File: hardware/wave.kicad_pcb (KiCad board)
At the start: 4 copper layers, 60 x 60 mm, 123 parts, among them J101 WAGO 2065-100, J102 WAGO 2065-100, J103 Cortex, J104 WAGO 2065-100, J105 WAGO 2065-100, J106 WAGO 2065-100, J107 WAGO 2065-100, J301 2x05_Horizontal, J401 2x05_Horizontal, J501 WAGO 2065-100, J502 WAGO 2065-100, Q201 IRF9358, SW101 SKSG, SW102 SKSG, U101 ATSAMD51J, U102 TPS78433QWDRBRQ1, U201 MA12070P, U301 THVD2442, U401 THVD2442, U501 74AHC1G125, Y101 32k768

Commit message: Update Library
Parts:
- FB101: value 47 Ohm -> ~
- FB201, FB202, FB203, FB204: value 50 Ohm -> ~
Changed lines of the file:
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@@
 			)
 		)
-		(property "Value" "50 Ohm"
+		(property "Value" "~"
 			(at 0 1.9 90)
 			(layer "F.Fab")
@@
 			)
 		)
-		(property "Value" "47 Ohm"
+		(property "Value" "~"
 			(at 0 2.9 0)
 			(layer "F.Fab")
@@
 			)
 		)
-		(property "Value" "50 Ohm"
+		(property "Value" "~"
 			(at 0 1.9 90)
 			(layer "F.Fab")
@@
 			)
 		)
-		(property "Value" "50 Ohm"
+		(property "Value" "~"
 			(at 0 1.9 90)
 			(layer "F.Fab")
@@
 		)
 		(group ""
-			(members "4532dc4e-f69d-412b-bc19-695d90100dcb" "8f0d22e3-918a-451d-a4a3-d23b9b599883"
-				"ae9bfc19-817d-4f4b-b84f-b22dd92c01e5" "bdaa4d0f-ab94-4c16-8f20-3c5ec3e83d21"
-				"f26a1357-79ae-4b96-a7f4-25831135af06"
+			(members "817afe4d-3ef8-4f34-841e-a1e0d13acd88" "8d5b3521-d299-4149-812d-e93ed26aa732"
+				"add876ea-4949-4e26-8186-7559bdf5a9eb" "b58fdfc9-b605-4197-b451-9f65004c44a9"
+				"c6308024-9361-453b-adb7-b5cdd279d357"
 			)
 		)
 		(group ""
-			(members "17461222-e6b8-4a40-a234-68067f321262" "96fa0783-c83b-424a-9582-f57065f0b73f"
-				"9e55e1cf-c869-4549-9032-91aab361908b" "9ef00dd0-bc50-46b7-b0af-3ca977389725"
-				"dabd2c8a-06ea-4384-a9f6-28d395331438"
+			(members "3d585795-267e-4acf-9233-fa6d3d19a673" "a58be4f5-7508-488d-900a-1671a0babb7c"
+				"bce2bd36-7243-4190-8a23-6d6964d44d4c" "e52a77fc-53a3-4bee-8404-ef76a262d8b0"
+				"fb6306f7-0653-42ec-a4a8-a7408847cb8f"
 			)
 		)
@@
 			)
 		)
-		(property "Value" "50 Ohm"
+		(property "Value" "~"
 			(at 0 1.9 90)
 			(layer "F.Fab")

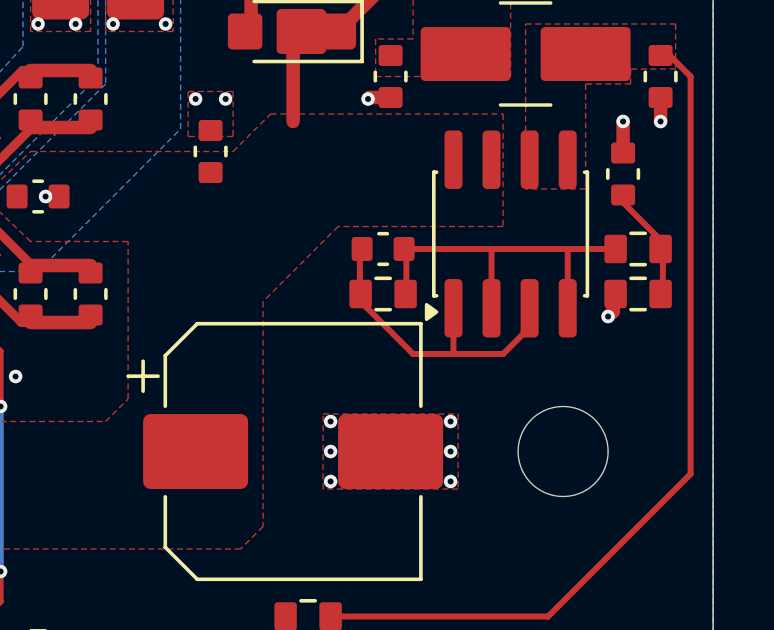
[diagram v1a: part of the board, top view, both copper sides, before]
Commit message: Update
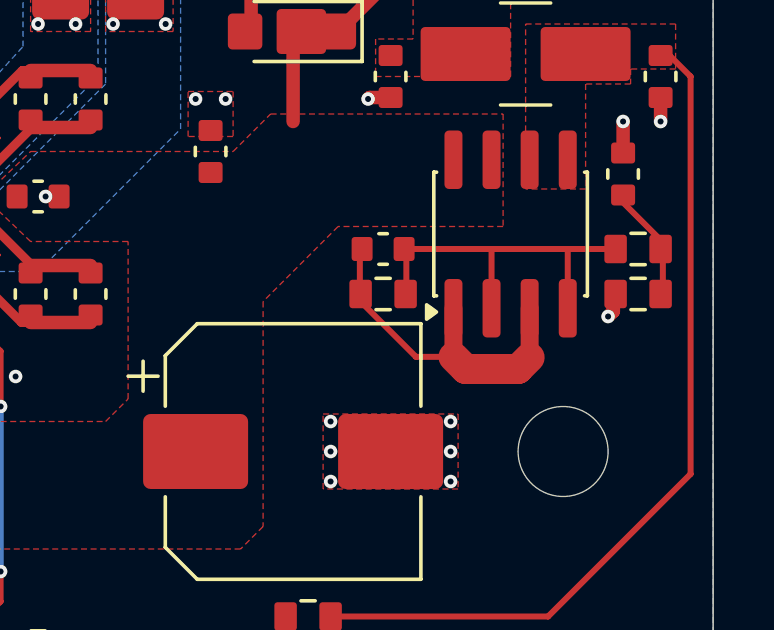
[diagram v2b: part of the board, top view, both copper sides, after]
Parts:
- FB101: value ~ -> 47 Ω
- FB201, FB202, FB203, FB204: value ~ -> 50 Ω
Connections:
- net /Amplifier Audio/PVDD renamed /Amplifier Audio/+PVDD
- net Net-(Q201A-G1) renamed /Amplifier Audio/Gate
- net Net-(Q201A-S1) renamed /Amplifier Audio/Source
- C105 pad 1: /+24V-Supply -> /+24V
- C106 pad 1: /Power -> /+24V-Supply
- FB101 pad 1: /+24V-Supply -> /+24V
- FB101 pad 2: /Power -> /+24V-Supply
- J101 pad 1: /+24V-Supply -> /+24V
- Q201 pad 5: /Power -> /+24V-Supply
- Q201 pad 6: /Power -> /+24V-Supply
- R101 pad 1: /Power -> /+24V-Supply
- TVS101 pad 2: /+24V-Supply -> /+24V
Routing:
- net /Power: track 28.4 -> 0.00 mm
- net /+24V-Supply: track 0.00 -> 28.4 mm
- net /Amplifier Audio/Source: track 10.8 -> 12.4 mm
- added copper zone on F.Cu, net /+24V
- removed copper zone on F.Cu, net /Power
